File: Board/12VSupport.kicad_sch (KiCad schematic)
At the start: 42 parts, among them J1 12V, J2 BATT, J3 BUCK_IN, J4 BUCK_OUT, J5 BOOST_IN, J6 BOOST_OUT, J8 HEATER, K1 SLA-05VDC-SL-C, K2 SLA-05VDC-SL-C, K3 SLA-05VDC-SL-C, K4 SLA-05VDC-SL-C, Q1 IRLML2502, Q2 IRLML2502, Q3 IRLML2502, Q4 IRLR7843, Q5 NCE30P30K, Q6 BSS138, U1 LM2596S-5, U4 ACS712xLCTR-20A

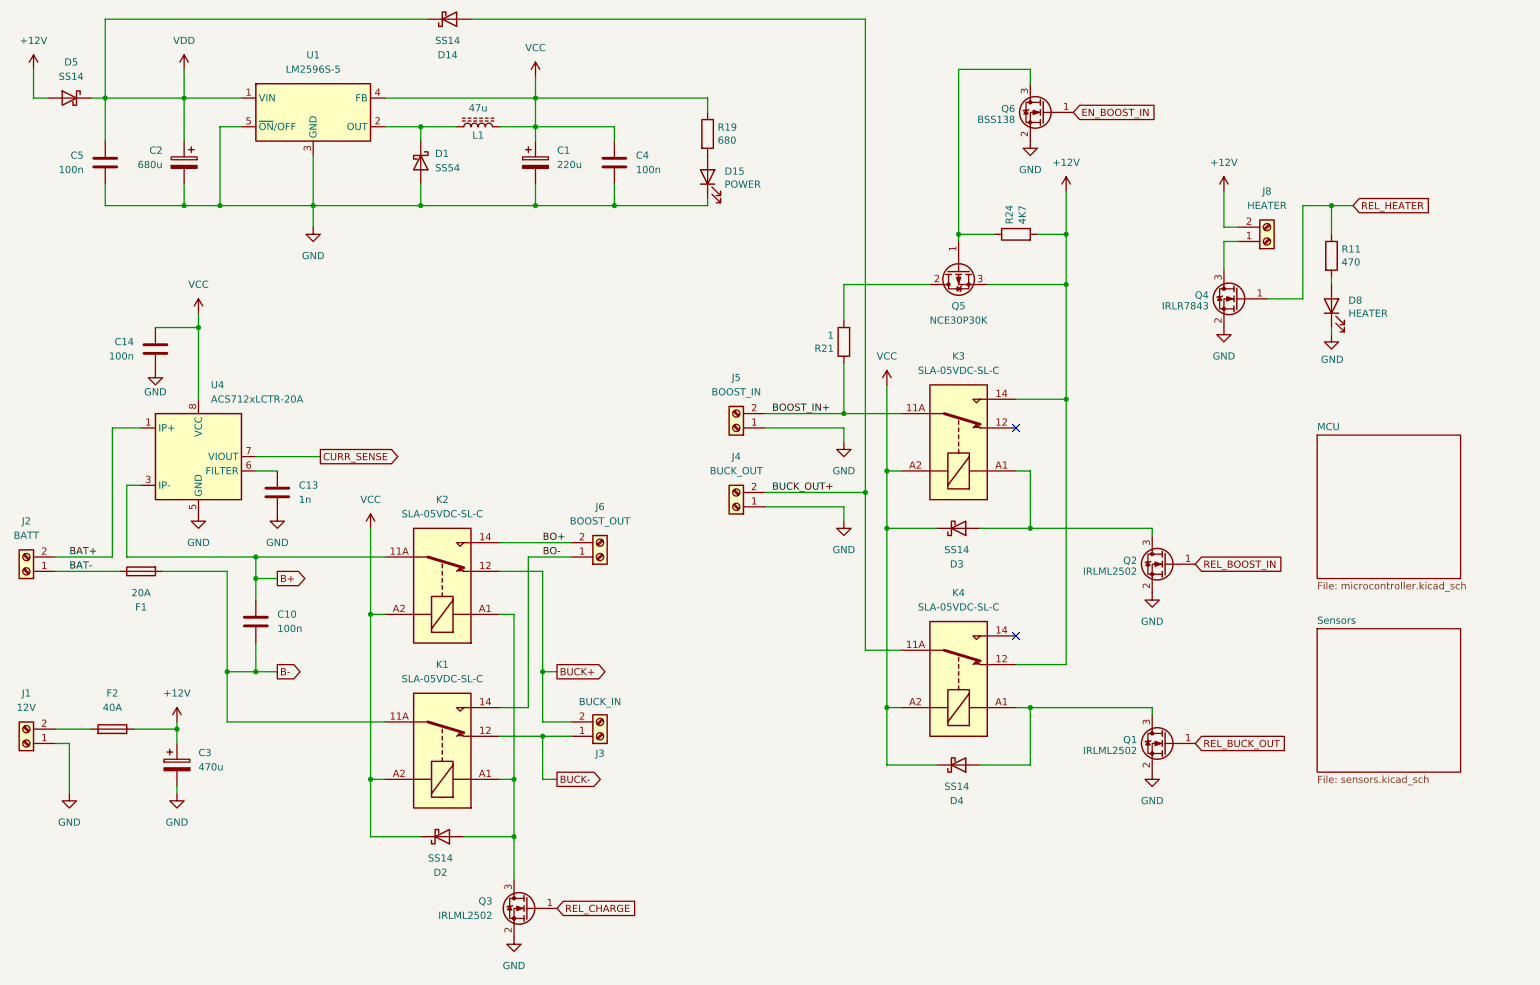
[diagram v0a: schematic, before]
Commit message: Bugfixes
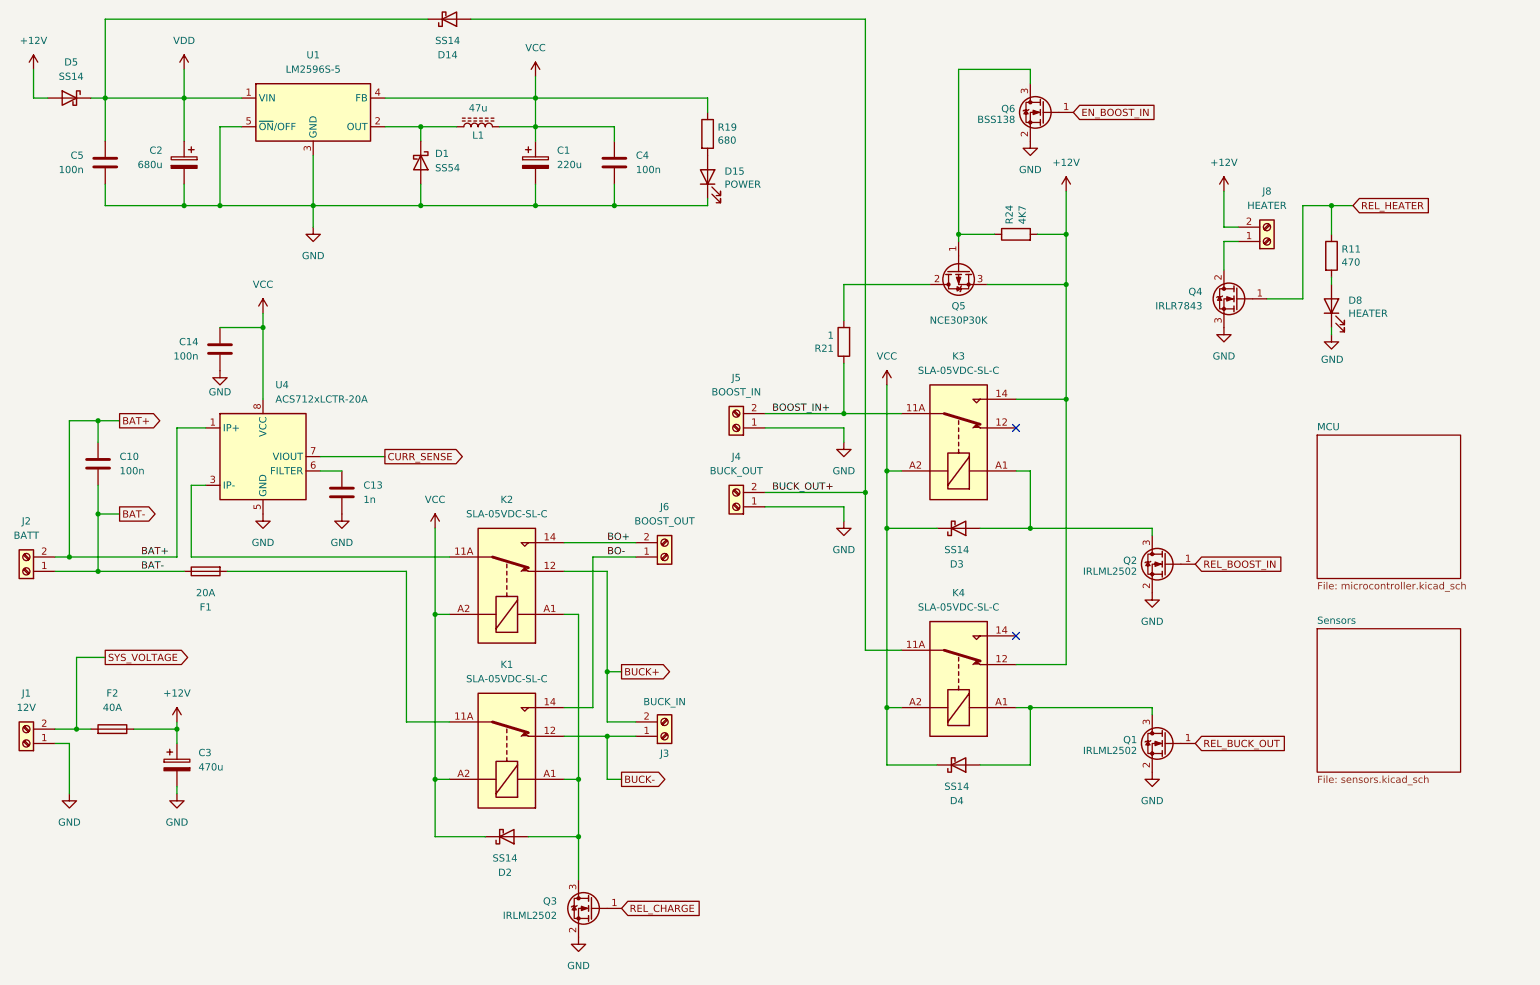
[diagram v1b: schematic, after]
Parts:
- removed Q4: IRLR7843, Package_TO_SOT_SMD:TO-252-2, symbol Transistor_FET:BSS138
- added Q4: IRLR7843, Package_TO_SOT_SMD:TO-252-2, symbol Transistor_FET:STD7NK40Z
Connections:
- net BAT+: now also C10.1
- net BAT-: now also C10.2
- net GND: now also Q4.3 (S)
- net REL_HEATER: now also Q4.1 (G)
- net SYS_VOLTAGE: now reaches F2.2, J1.2 (Pin_2)
- net at J8.1 (Pin_1): now also Q4.2 (D)
- net B+: no longer names the net of K2.11A, K2.11B, U4.3 (IP-), U4.4 (IP-)
- net B+: no longer C10.1
- net B-: no longer names the net of F1.2, K1.11A, K1.11B
- net B-: no longer C10.2
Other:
- moved on the sheet: C10, C13, C14, D2, F1, J3, J6, K1, K2, Q3, U4
